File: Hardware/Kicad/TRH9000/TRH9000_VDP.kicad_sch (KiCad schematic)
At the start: 13 parts, among them U1 V9990, U2 KM428C256, U3 KM428C256, X1 14.31818MHz, Y1 21.47727Mhz

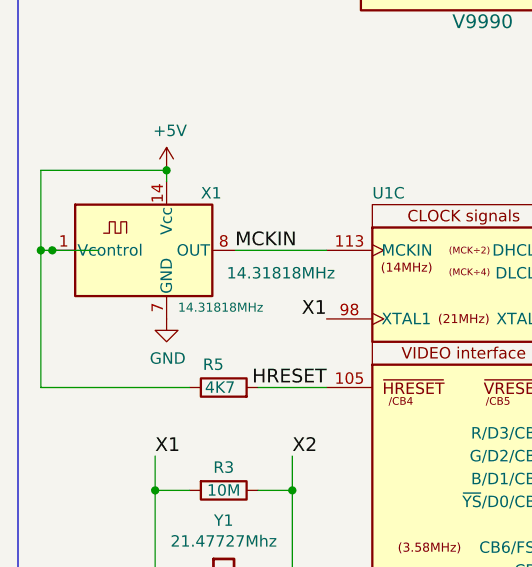
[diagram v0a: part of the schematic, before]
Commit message: Routing, readme, etc
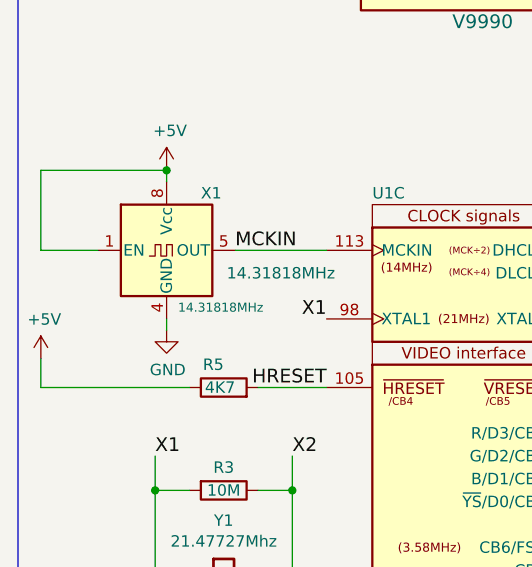
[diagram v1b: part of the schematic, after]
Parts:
- X1: footprint Oscillator:Oscillator_DIP-14 -> Oscillator:Oscillator_DIP-8; symbol Oscillator:OCXO-14 -> Oscillator:CXO_DIP8
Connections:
- net +5V: now also X1.8 (Vcc); no longer X1.14 (Vcc)
- net GND: now also X1.4 (GND); no longer X1.7 (GND)
- net MCKIN: now also X1.5 (OUT); no longer X1.8 (OUT)
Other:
- moved on the sheet: X1
